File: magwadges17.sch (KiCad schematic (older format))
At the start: 15 parts, among them J1 PGM, J2 JACK_2P, U1 ATTINY861A-SU

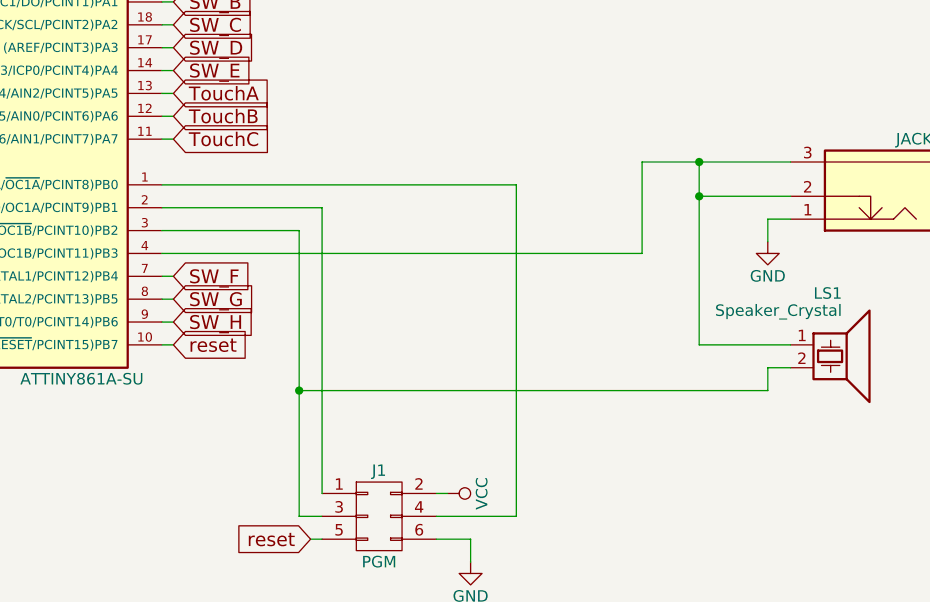
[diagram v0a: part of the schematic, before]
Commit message: Update wadges
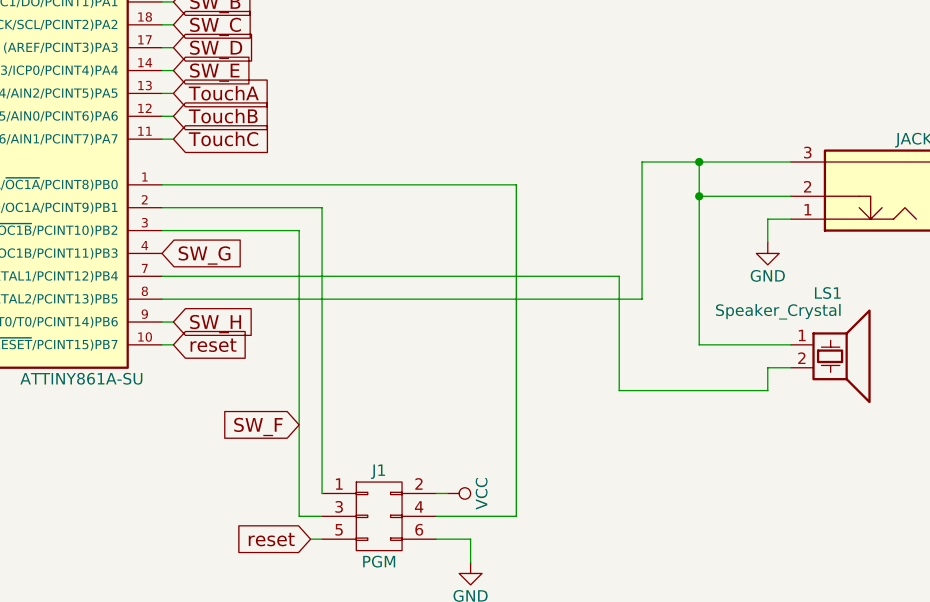
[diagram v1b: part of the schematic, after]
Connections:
- net SW_F: now also J1.3 (P3), U1.3 ((SCK/USCK/SCL/~OC1B~/PCINT10)PB2); no longer U1.7 ((ADC7/~OC1D~/CLKI/XTAL1/PCINT12)PB4)
- net SW_G: now also U1.4 ((OC1B/PCINT11)PB3); no longer U1.8 ((ADC8/OC1D/CLKO/XTAL2/PCINT13)PB5)
- net at J2.2, J2.3, LS1.1: now also U1.8 ((ADC8/OC1D/CLKO/XTAL2/PCINT13)PB5); no longer U1.4 ((OC1B/PCINT11)PB3)
- new net: LS1.2, U1.7 ((ADC7/~OC1D~/CLKI/XTAL1/PCINT12)PB4)
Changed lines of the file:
@@
 Text GLabel 5200 1650 2    60   Input ~ 0
 SW_E
-Text GLabel 5200 2550 2    60   Input ~ 0
+Text GLabel 5750 3200 0    60   Input ~ 0
 SW_F
-Text GLabel 5200 2650 2    60   Input ~ 0
+Text GLabel 5150 2450 2    60   Input ~ 0
 SW_G
 Text GLabel 5200 2750 2    60   Input ~ 0
@@
 	5200 1950 5150 1950
 Wire Wire Line
-	5150 2550 5200 2550
-Wire Wire Line
-	5200 2650 5150 2650
+	5150 2550 7150 2550
+Wire Wire Line
+	7250 2650 5150 2650
 Wire Wire Line
 	5150 2750 5200 2750
@@
 	5850 2250 5150 2250
 Wire Wire Line
-	5150 2450 7250 2450
-Wire Wire Line
-	7250 2450 7250 2050
+	7250 2050 7250 2650
 Wire Wire Line
 	7250 2050 7900 2050
@@
 	1    0    0    -1
 $EndComp
-Wire Wire Line
-	7800 3050 5750 3050
-Connection ~ 5750 3050
 Text GLabel 7750 5250 3    60   Input ~ 0
 reset
+Wire Wire Line
+	7150 2550 7150 3050
+Wire Wire Line
+	7150 3050 7800 3050
 $EndSCHEMATC

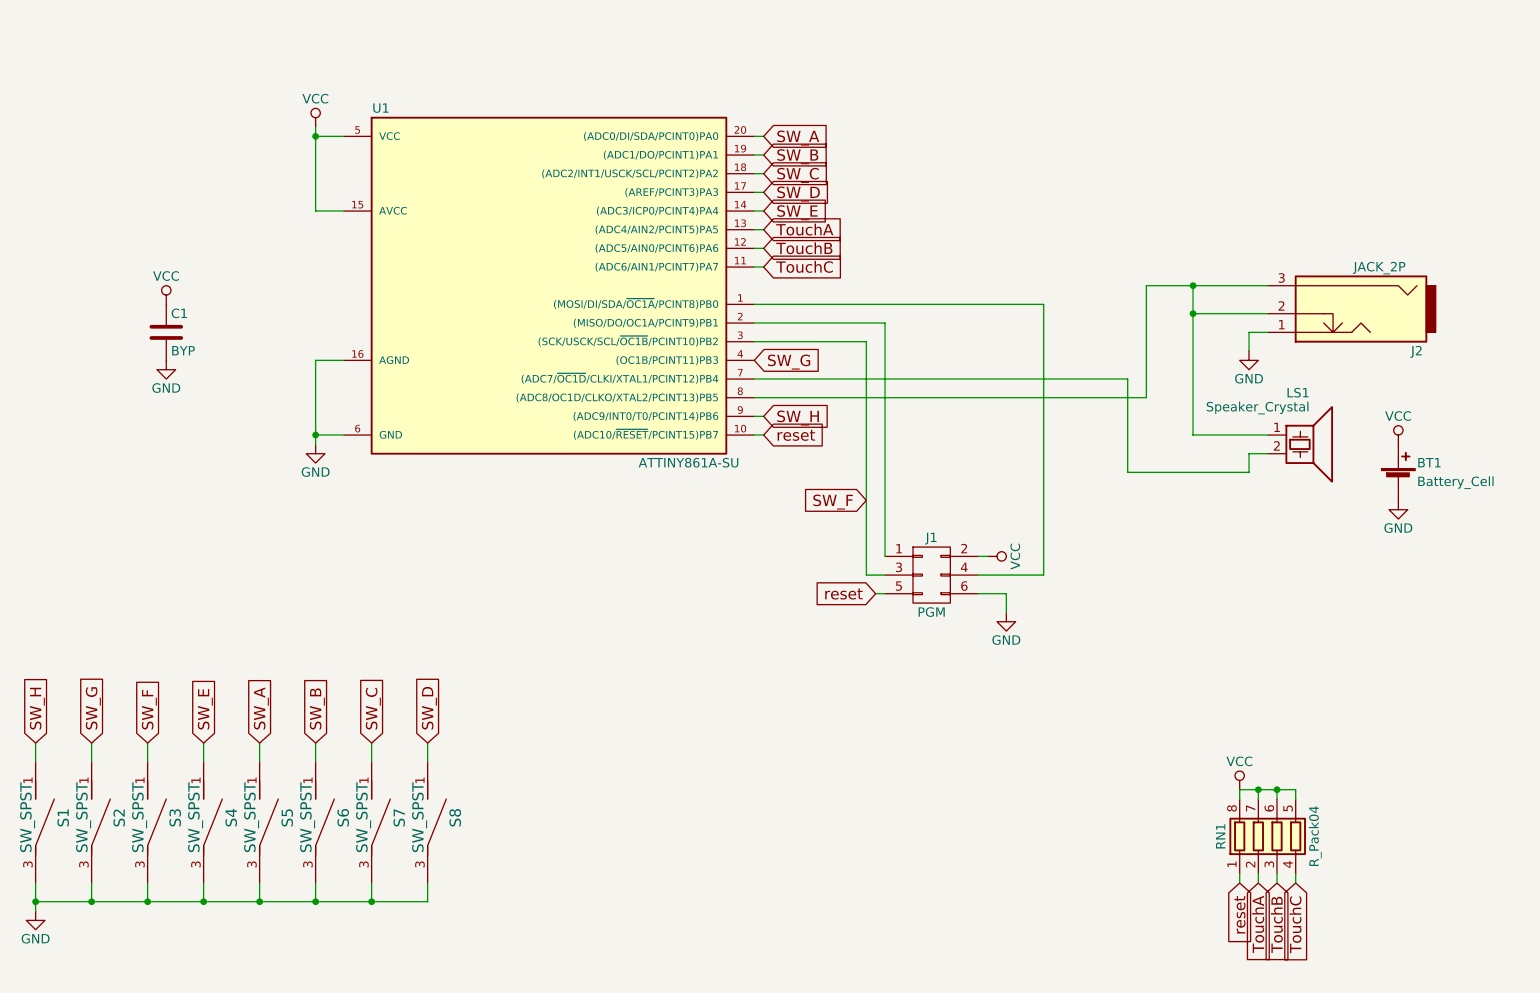
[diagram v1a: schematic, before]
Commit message: Update design
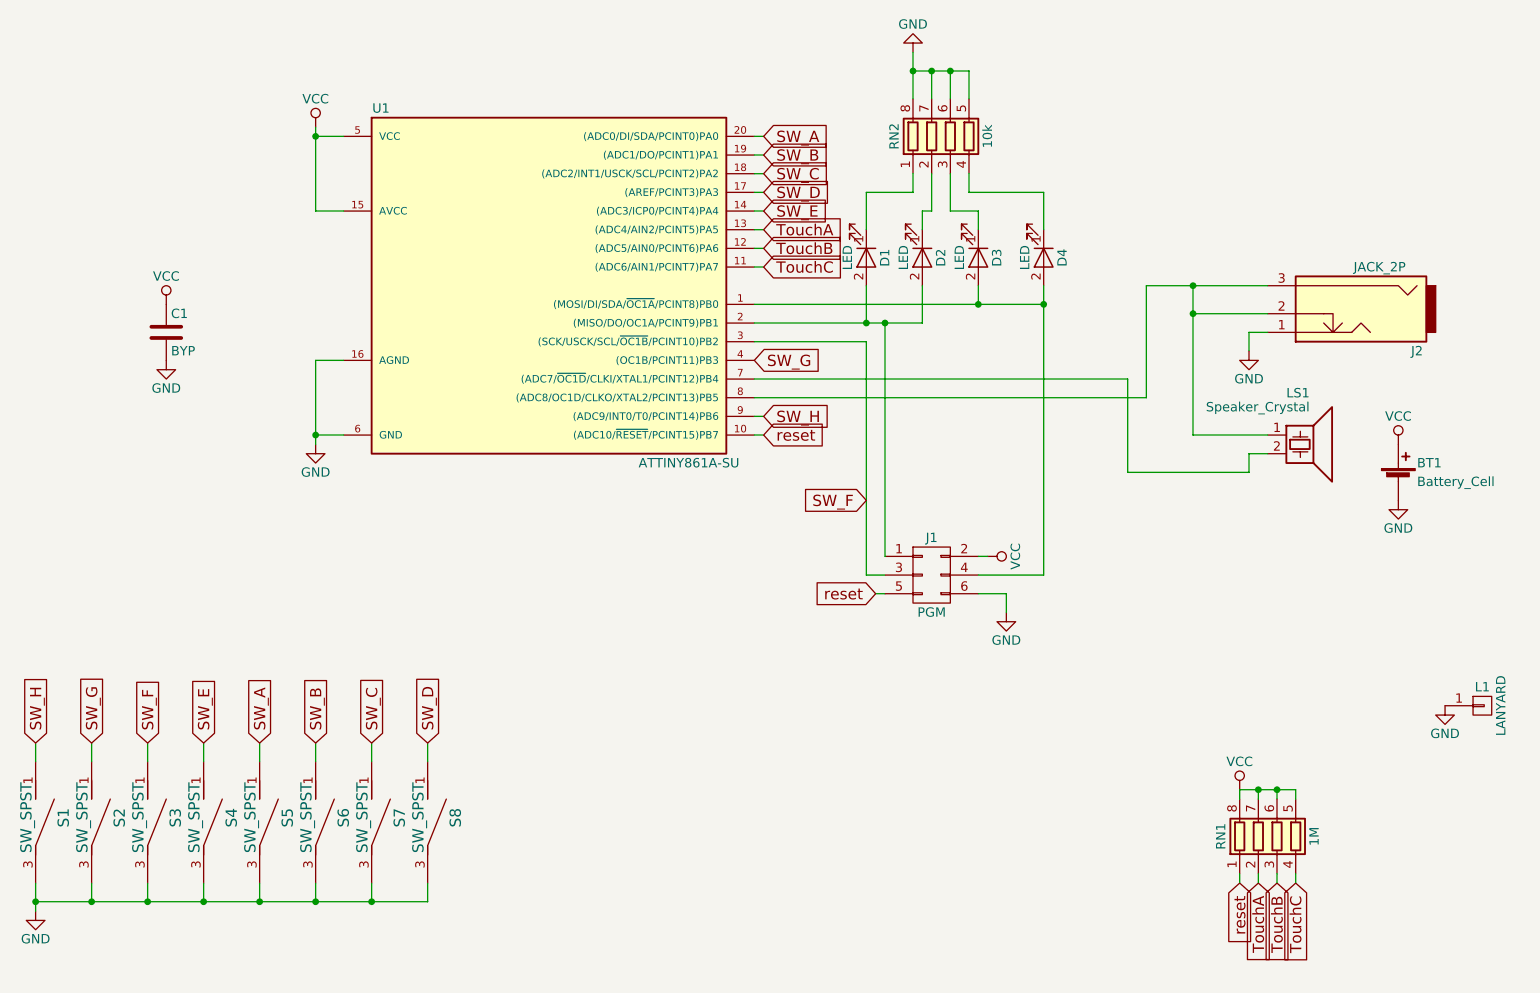
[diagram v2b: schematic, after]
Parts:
- added D1, D2, D3, D4: LED, SM0805, symbol LED
- added L1: LANYARD, 1pin, symbol CONN_01X01
- added RN2: 10k, NETWORK1206, symbol R_Pack04
- RN1: value R_Pack04 -> 1M
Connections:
- net GND: now also L1.1 (P1), RN2.5 (R4.2), RN2.6 (R3.2), RN2.7 (R2.2), RN2.8 (R1.2)
- net at J1.1 (P1), U1.2 ((MISO/DO/OC1A/PCINT9)PB1): now also D1.2 (A), D2.2 (A)
- net at J1.4 (P4), U1.1 ((MOSI/DI/SDA/~OC1A~/PCINT8)PB0): now also D3.2 (A), D4.2 (A)
- new net: D4.1 (K), RN2.4 (R4.1)
- new net: D3.1 (K), RN2.3 (R3.1)
- new net: D2.1 (K), RN2.2 (R2.1)
- new net: D1.1 (K), RN2.1 (R1.1)
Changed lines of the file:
@@
 P 7950 5000
 F 0 "RN1" V 7650 5000 50  0000 C CNN
-F 1 "R_Pack04" V 8150 5000 50  0000 C CNN
+F 1 "1M" V 8150 5000 50  0000 C CNN
 F 2 "NETWORK1206" V 8225 5000 50  0001 C CNN
 F 3 "" H 7950 5000 50  0001 C CNN
@@
 	5150 2150 6700 2150
 Wire Wire Line
-	6700 2150 6700 3600
+	6700 2050 6700 3600
 Wire Wire Line
 	6700 3600 6350 3600
@@
 	5750 3600 5850 3600
 Wire Wire Line
-	5850 2250 5150 2250
+	5150 2250 6050 2250
 Wire Wire Line
 	7250 2050 7250 2650
@@
 Wire Wire Line
 	7150 3050 7800 3050
+$Comp
+L CONN_01X01 L1
+U 1 1 5982C11E
+P 9050 4300
+F 0 "L1" H 9050 4400 50  0000 C CNN
+F 1 "LANYARD" V 9150 4300 50  0000 C CNN
+F 2 "1pin" H 9050 4300 50  0001 C CNN
+F 3 "" H 9050 4300 50  0001 C CNN
+	1    9050 4300
+	1    0    0    -1
+$EndComp
+Wire Wire Line
+	5750 2250 5750 2050
+Connection ~ 5750 2250
+Wire Wire Line
+	6050 2250 6050 2050
+Connection ~ 5850 2250
+Wire Wire Line
+	6350 2050 6350 2150
+Connection ~ 6350 2150
+Connection ~ 6700 2150
+$Comp
+L R_Pack04 RN2
+U 1 1 5982CF21
+P 6200 1250
+F 0 "RN2" V 5900 1250 50  0000 C CNN
+F 1 "10k" V 6400 1250 50  0000 C CNN
+F 2 "NETWORK1206" V 6475 1250 50  0001 C CNN
+F 3 "" H 6200 1250 50  0001 C CNN
+	1    6200 1250
+	1    0    0    -1
+$EndComp
+Wire Wire Line
+	6700 1550 6700 1750
+Wire Wire Line
+	6300 1550 6700 1550
+Wire Wire Line
+	6300 1450 6300 1550
+Wire Wire Line
+	6350 1650 6350 1750
+Wire Wire Line
+	6200 1650 6350 1650
+Wire Wire Line
+	6200 1450 6200 1650
+Wire Wire Line
+	6050 1650 6050 1750
+Wire Wire Line
+	6100 1650 6050 1650
+Wire Wire Line
+	6100 1450 6100 1650
+Wire Wire Line
+	5750 1550 5750 1750
+Wire Wire Line
+	6000 1550 5750 1550
+Wire Wire Line
+	6000 1450 6000 1550
+$Comp
+L LED D4
+U 1 1 5982C740
+P 6700 1900
+F 0 "D4" H 6700 2000 50  0000 C CNN
+F 1 "LED" H 6700 1800 50  0000 C CNN
+F 2 "SM0805" H 6700 1900 50  0001 C CNN
+F 3 "" H 6700 1900 50  0001 C CNN
+	1    6700 1900
+	0    1    1    0
+$EndComp
+$Comp
+L LED D3
+U 1 1 5982C999
+P 6350 1900
+F 0 "D3" H 6350 2000 50  0000 C CNN
+F 1 "LED" H 6350 1800 50  0000 C CNN
+F 2 "SM0805" H 6350 1900 50  0001 C CNN
+F 3 "" H 6350 1900 50  0001 C CNN
+	1    6350 1900
+	0    1    1    0
+$EndComp
+$Comp
+L LED D2
+U 1 1 5982C9EB
+P 6050 1900
+F 0 "D2" H 6050 2000 50  0000 C CNN
+F 1 "LED" H 6050 1800 50  0000 C CNN
+F 2 "SM0805" H 6050 1900 50  0001 C CNN
+F 3 "" H 6050 1900 50  0001 C CNN
+	1    6050 1900
+	0    1    1    0
+$EndComp
+$Comp
+L LED D1
+U 1 1 5982CA40
+P 5750 1900
+F 0 "D1" H 5750 2000 50  0000 C CNN
+F 1 "LED" H 5750 1800 50  0000 C CNN
+F 2 "SM0805" H 5750 1900 50  0001 C CNN
+F 3 "" H 5750 1900 50  0001 C CNN
+	1    5750 1900
+	0    1    1    0
+$EndComp
+Wire Wire Line
+	6000 800  6000 1050
+Wire Wire Line
+	6000 900  6300 900
+Wire Wire Line
+	6300 900  6300 1050
+Wire Wire Line
+	6200 1050 6200 900
+Connection ~ 6200 900
+Wire Wire Line
+	6100 900  6100 1050
+Connection ~ 6100 900
+Connection ~ 6000 900
+$Comp
+L GND #PWR012
+U 1 1 5982DE9F
+P 6000 800
+F 0 "#PWR012" H 6000 550 50  0001 C CNN
+F 1 "GND" H 6000 650 50  0000 C CNN
+F 2 "" H 6000 800 50  0001 C CNN
+F 3 "" H 6000 800 50  0001 C CNN
+	1    6000 800
+	-1   0    0    1
+$EndComp
+$Comp
+L GND #PWR013
+U 1 1 5982E2EC
+P 8850 4300
+F 0 "#PWR013" H 8850 4050 50  0001 C CNN
+F 1 "GND" H 8850 4150 50  0000 C CNN
+F 2 "" H 8850 4300 50  0001 C CNN
+F 3 "" H 8850 4300 50  0001 C CNN
+	1    8850 4300
+	1    0    0    -1
+$EndComp
 $EndSCHEMATC
